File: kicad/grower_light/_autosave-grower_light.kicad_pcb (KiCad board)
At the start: 2 copper layers, 98 x 41 mm, 34 parts, among them J1 AC, J2 AC_IN, J3 PWR_+5V, J4 OUTPUT, J6 ESP_UART, J7 Sensors, Q1 BT139-600, Q2 BSS138, Q3 BSS138, SW1 RESET, U1 MOC3023M, U2 LD1117S33TR_SOT223, U3 ESP-12_07v2

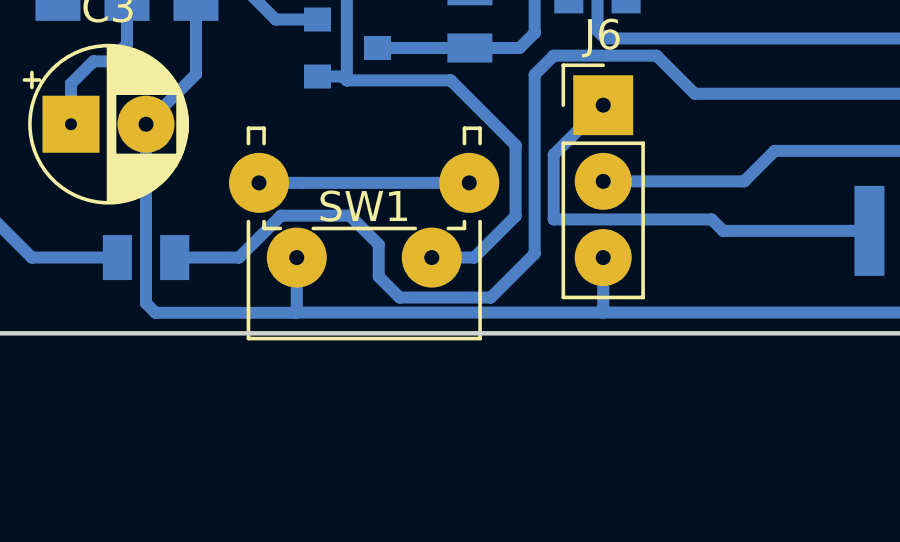
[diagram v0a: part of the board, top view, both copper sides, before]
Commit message: Final pcb
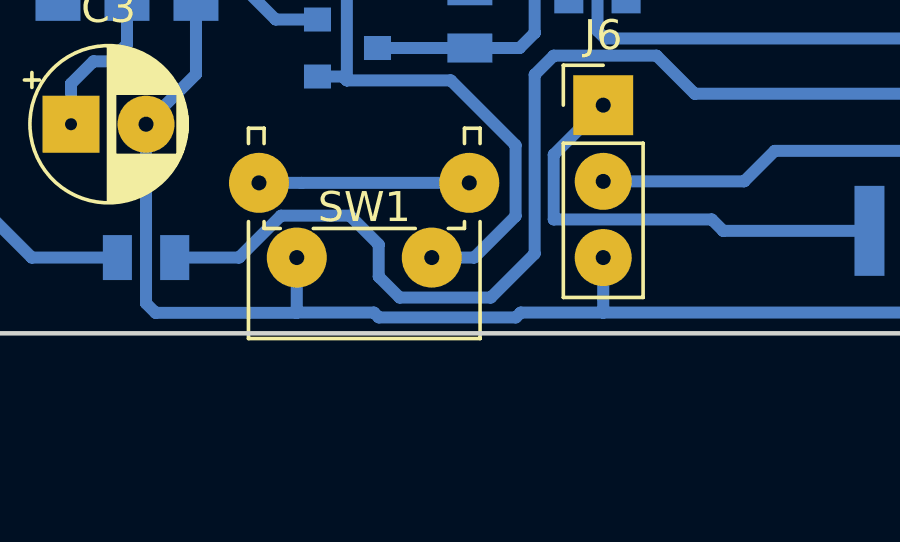
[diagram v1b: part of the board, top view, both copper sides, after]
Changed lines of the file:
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@@
     (thickness 1.6)
     (drawings 9)
-    (tracks 269)
+    (tracks 273)
     (zones 0)
     (modules 34)
@@
     (46 B.CrtYd user)
     (47 F.CrtYd user)
-    (48 B.Fab user hide)
+    (48 B.Fab user)
     (49 F.Fab user)
   )
@@
   (segment (start 147.275 114.985) (end 148.689213 114.985) (width 0.4) (layer B.Cu) (net 0))
   (segment (start 148.689213 114.985) (end 154.285 114.985) (width 0.4) (layer B.Cu) (net 0))
+  (segment (start 148.535 119.308) (end 151.108 119.308) (width 0.4) (layer B.Cu) (net 1))
+  (segment (start 151.108 119.308) (end 151.27099 119.47099) (width 0.4) (layer B.Cu) (net 1))
+  (segment (start 151.27099 119.47099) (end 155.83701 119.47099) (width 0.4) (layer B.Cu) (net 1))
+  (segment (start 155.83701 119.47099) (end 156 119.308) (width 0.4) (layer B.Cu) (net 1))
+  (segment (start 156 119.308) (end 158.75 119.308) (width 0.4) (layer B.Cu) (net 1))
   (segment (start 158.75 119.308) (end 181.555 119.308) (width 0.4) (layer B.Cu) (net 1))
   (segment (start 158.75 117.475) (end 158.75 118.818502) (width 0.4) (layer B.Cu) (net 1))
-  (segment (start 148.535 119.308) (end 158.75 119.308) (width 0.4) (layer B.Cu) (net 1))
   (segment (start 158.75 118.818502) (end 158.75 119.308) (width 0.4) (layer B.Cu) (net 1))
   (segment (start 181.555 119.308) (end 181.625 119.238) (width 0.4) (layer B.Cu) (net 1))
